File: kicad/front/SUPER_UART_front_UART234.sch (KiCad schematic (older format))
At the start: 63 parts, among them CON7 PORT A, CON8 PORT C, Q10 2N7002PS, Q11 N-MOS_small, Q7 PDTA143ZT, Q8 2N7002PS, Q9 PDTA143ZT, U11 74HC595D, U12 74LVC8T245PW, U13 74LVC2T45DCU, U14 74LVC1T45GW, U15 74LVC1T45GW, U16 LP2951CD

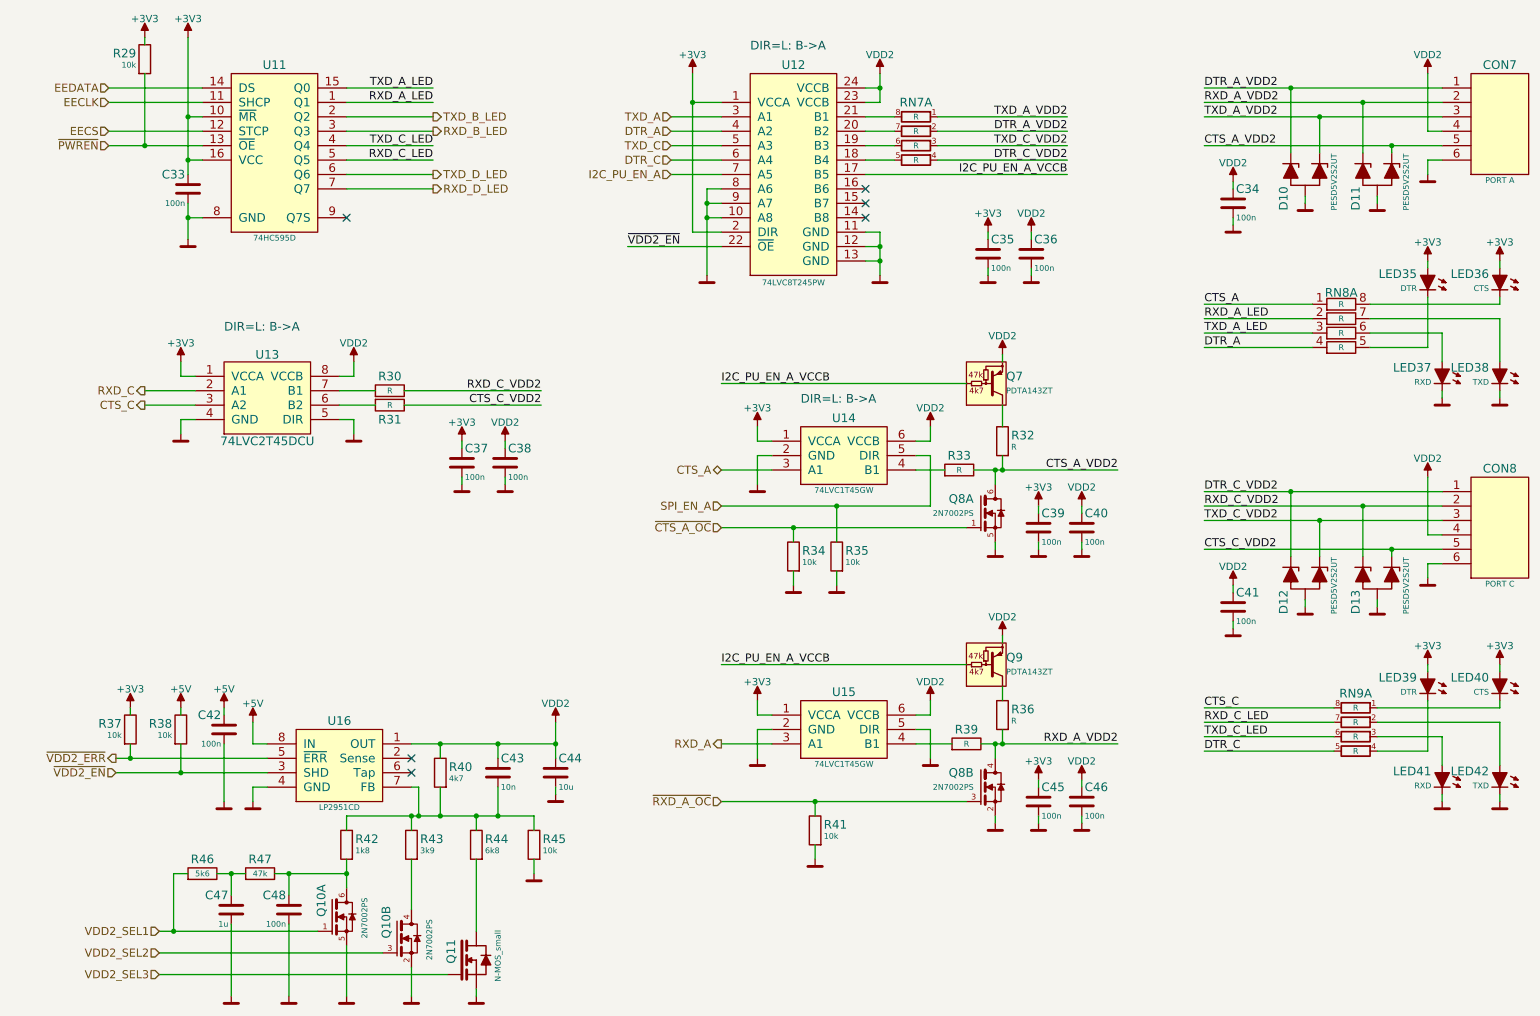
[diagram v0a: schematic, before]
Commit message: PCB placement
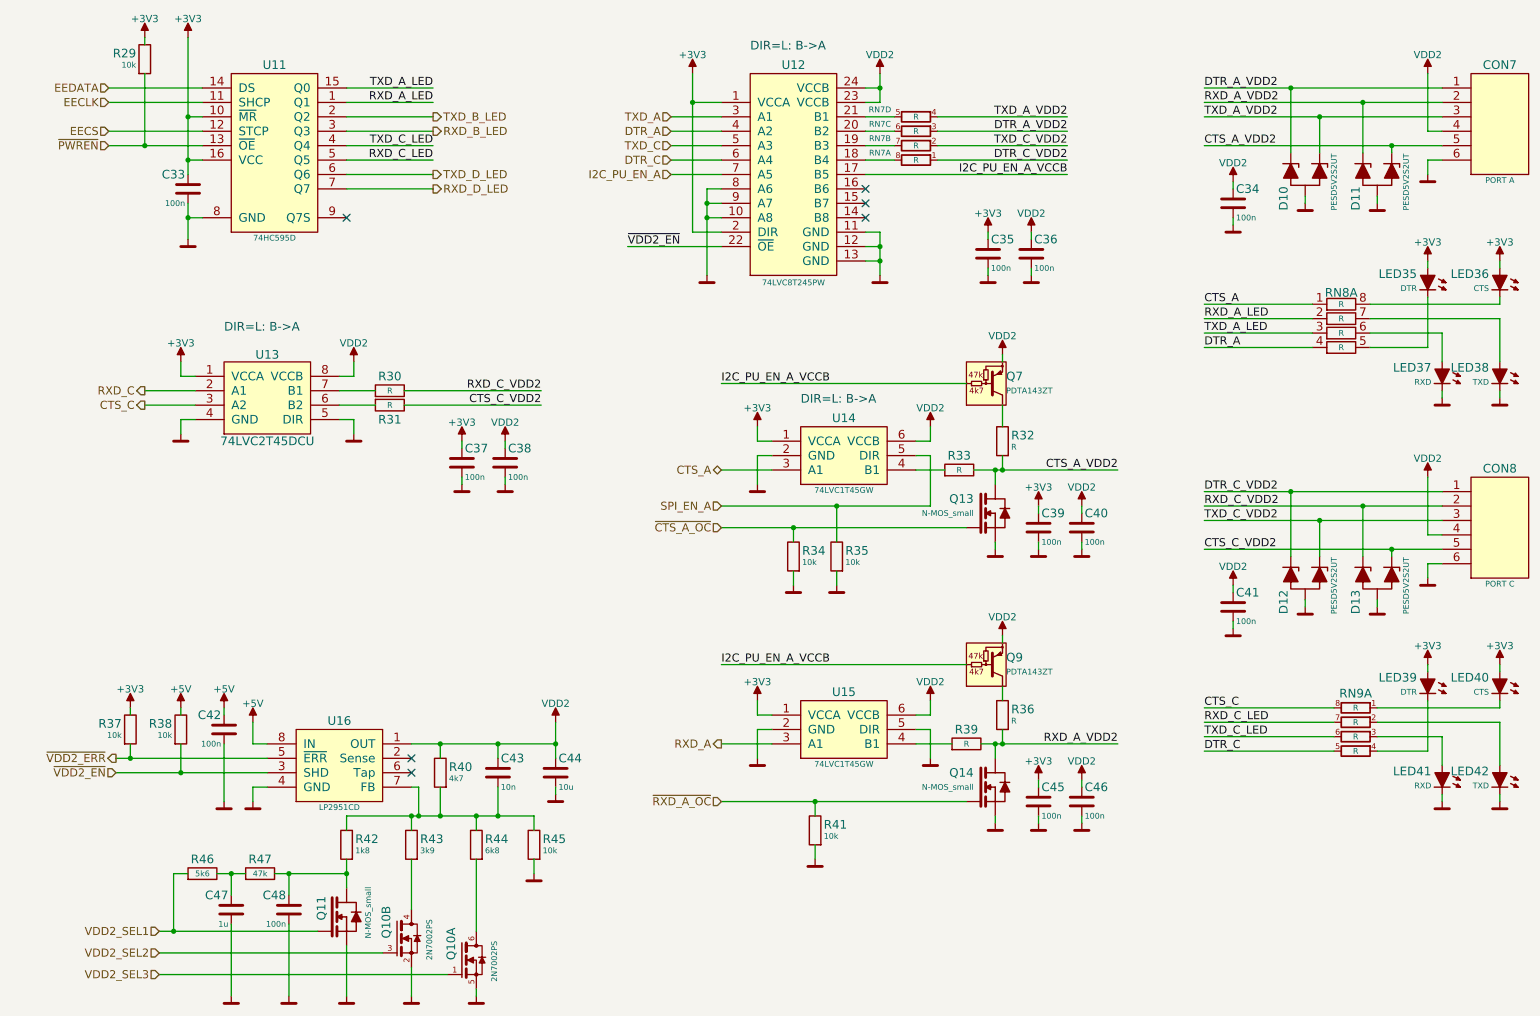
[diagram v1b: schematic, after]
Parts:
- removed Q8: 2N7002PS, niceSemiconductors:SC70-6_N, symbol 2N7002PS
- added Q13, Q14: N-MOS_small, SOT23-3_N, symbol N-MOS_small
- RN7, RN9: footprint pnRLC:4x0603_N -> niceRLC:4x0603_N
- RN8: footprint 4x0603_N -> niceRLC:4x0603_N
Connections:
- net CTS_A_VDD2: now also Q13.3 (D)
- net DTR_A_VDD2: now also RN7.3; no longer RN7.2
- net DTR_C_VDD2: now also RN7.1; no longer RN7.4
- net GND: now also Q13.2 (S), Q14.2 (S)
- net RXD_A_VDD2: now also Q14.3 (D)
- net TXD_A_VDD2: now also RN7.4; no longer RN7.1
- net TXD_C_VDD2: now also RN7.2; no longer RN7.3
- net VDD2_SEL1: now also Q11.1 (G); no longer Q10.1 (G)
- net VDD2_SEL3: now also Q10.1 (G); no longer Q11.1 (G)
- net ~CTS_A_OC: now also Q13.1 (G)
- net ~RXD_A_OC: now also Q14.1 (G)
- net at U12.18 (B4): now also RN7.8; no longer RN7.5
- net at U12.19 (B3): now also RN7.7; no longer RN7.6
- net at U12.20 (B2): now also RN7.6; no longer RN7.7
- net at U12.21 (B1): now also RN7.5; no longer RN7.8
- net at C48.1, R42.1, R47.2: now also Q11.3 (D); no longer Q10.6 (D)
- net at R44.1: now also Q10.6 (D); no longer Q11.3 (D)
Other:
- moved on the sheet: Q10A, Q11
